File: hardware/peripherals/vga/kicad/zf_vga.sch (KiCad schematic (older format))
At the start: 34 parts, among them J1 Conn_02x04_Odd_Even, J2 Conn_02x13_Odd_Even, J3 DB15_Female, J4 DB9_Male, J5 DB9_Male, SW1 SW_DIP_x03, U1 4040, U10 74HC165, U11 AS6C6264, U12 74HC541, U13 74HC541, U14 74HC541, U2 4040, U3 GAL16V8, U4 GAL16V8, U5 74HC541, U6 74HC541, U7 74HC00, U8 74HC04, U9 74HC74, X1 CXO_DIP14

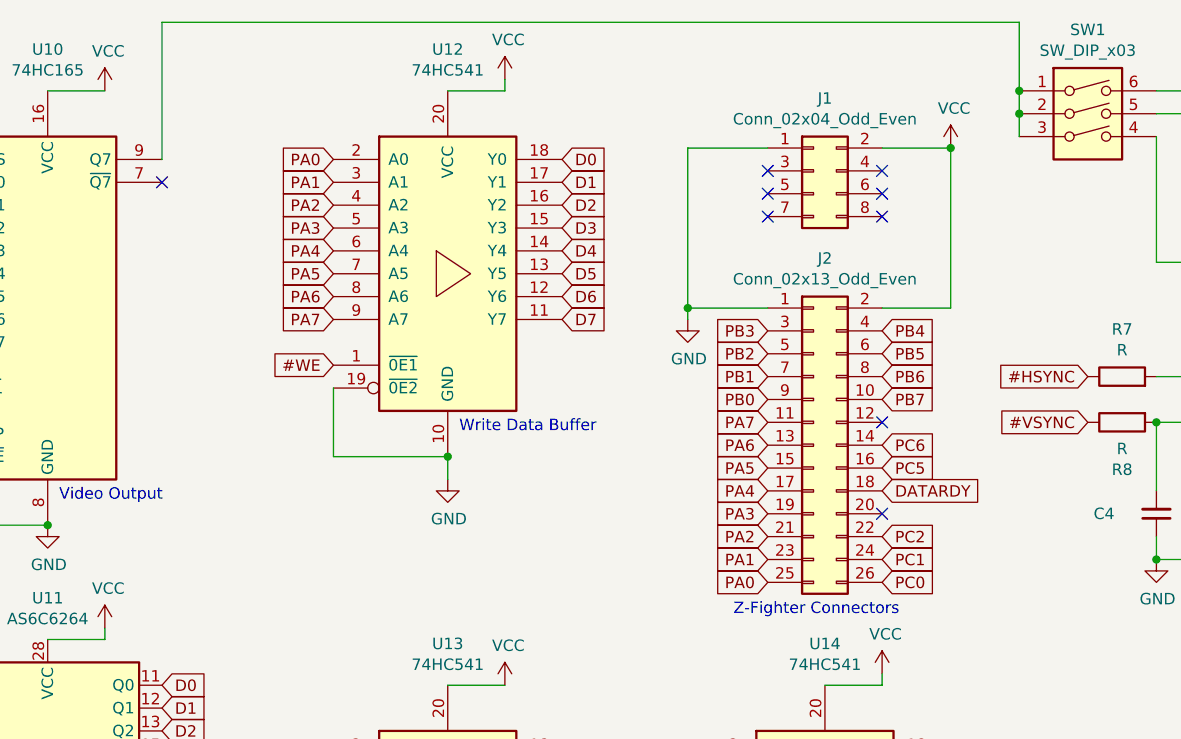
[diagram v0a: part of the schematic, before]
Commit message: Started PCB
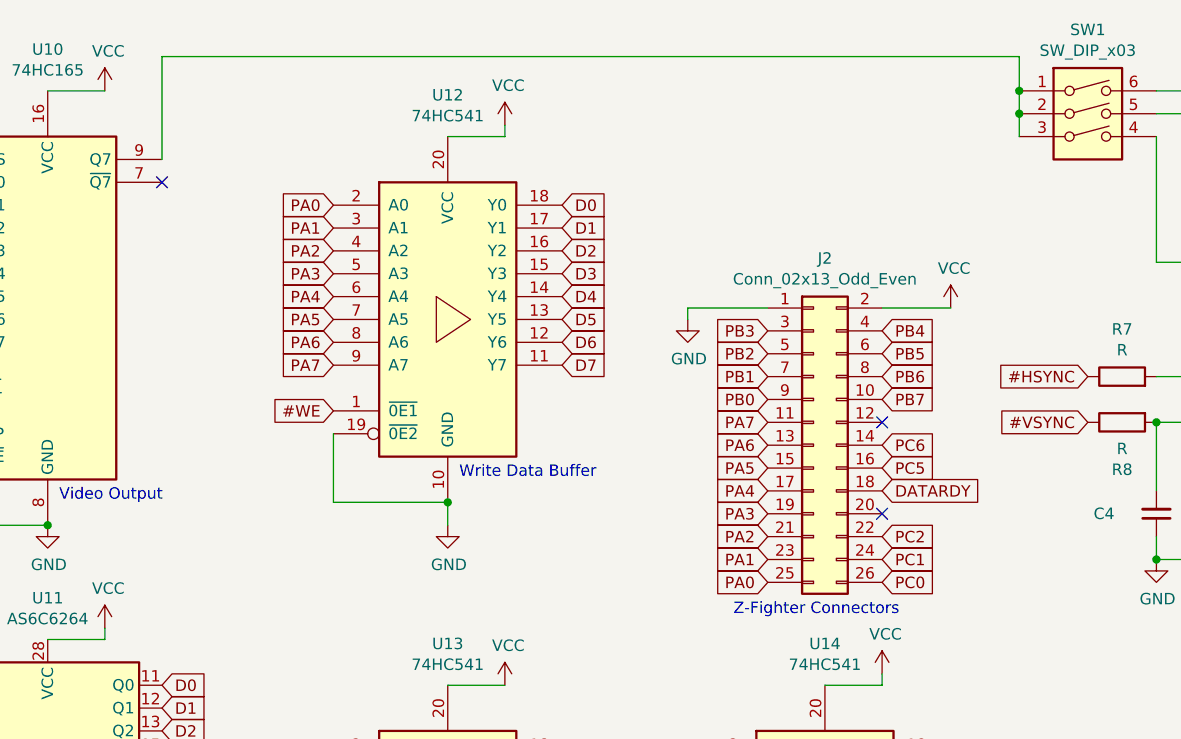
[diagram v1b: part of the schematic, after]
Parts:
- removed J1: Conn_02x04_Odd_Even, symbol Connector_Generic:Conn_02x04_Odd_Even
- C1, C2, C3, C4, C5: footprint (none) -> Capacitor_THT:C_Disc_D7.5mm_W2.5mm_P5.00mm
- J2: footprint (none) -> Connector_IDC:IDC-Header_2x13_P2.54mm_Vertical
- R1, R2, R3, R4, R5, R6, R7, R8: footprint (none) -> Resistor_THT:R_Axial_DIN0207_L6.3mm_D2.5mm_P7.62mm_Horizontal
- SW1: footprint (none) -> Button_Switch_THT:SW_DIP_SPSTx03_Slide_6.7x9.18mm_W7.62mm_P2.54mm_LowProfile
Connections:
- no-connect marks 35 -> 29
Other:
- moved on the sheet: U12

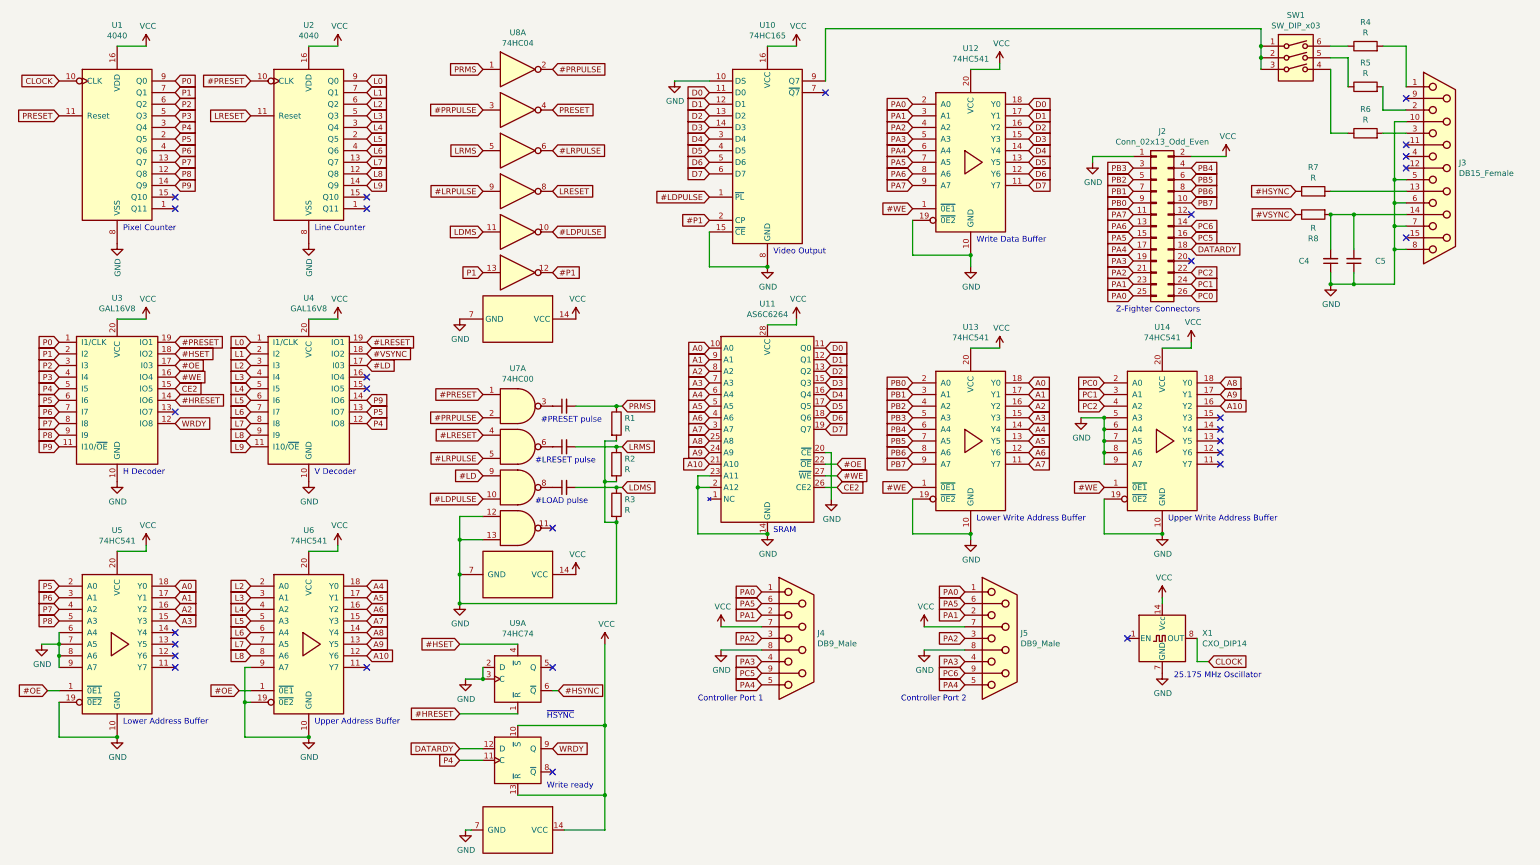
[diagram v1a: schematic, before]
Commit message: Bypass caps
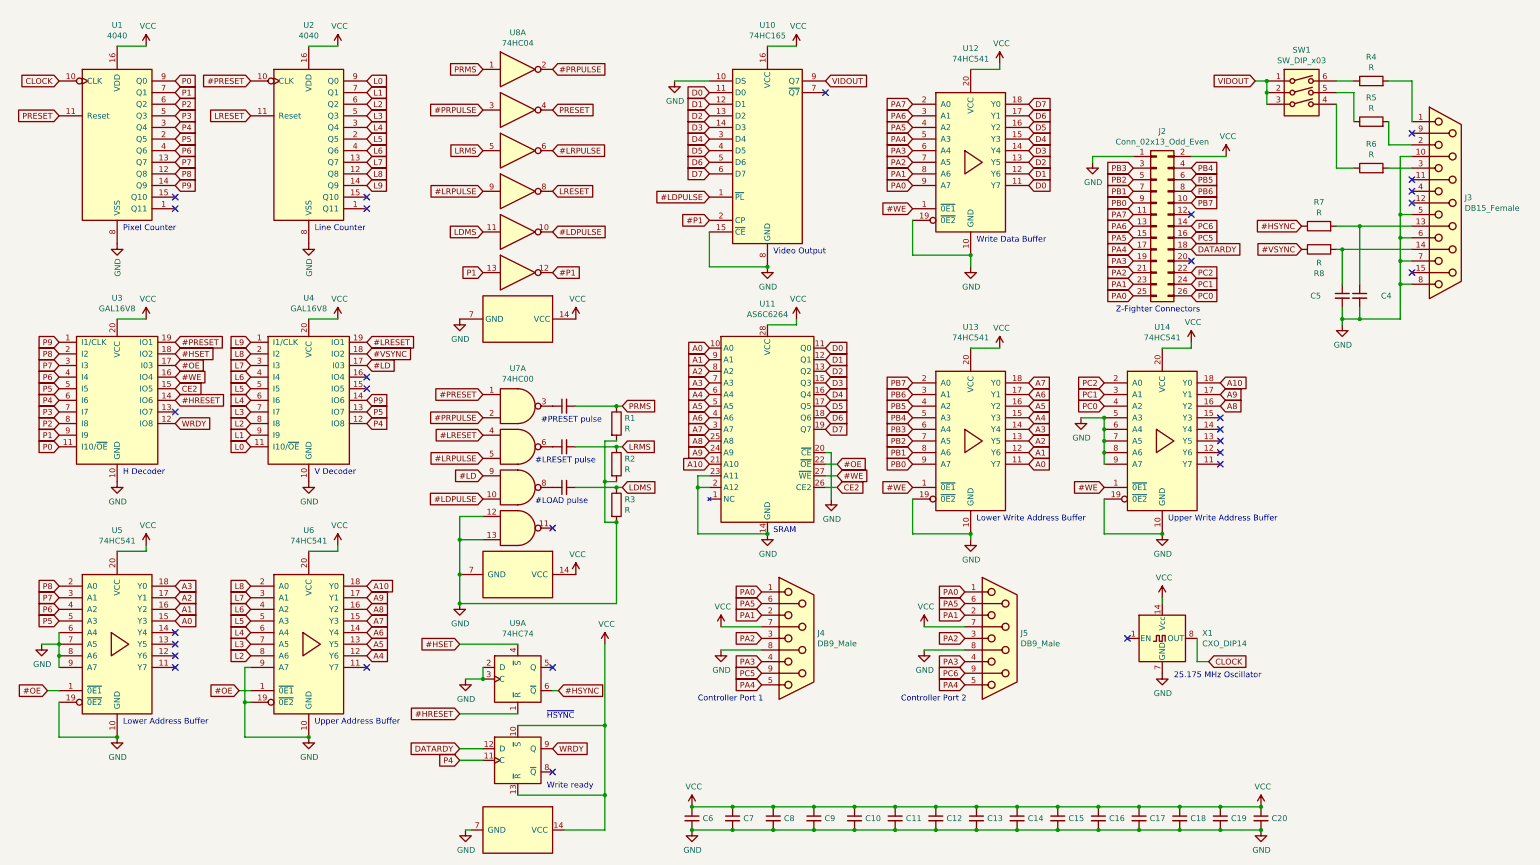
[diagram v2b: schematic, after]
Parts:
- added C10, C11, C12, C13, C14, C15, C16, C17, C18, C19, C20, C6, C7, C8, C9: 0.1uF, Capacitor_THT:C_Disc_D7.5mm_W2.5mm_P5.00mm, symbol Device:C_Small
- SW1: footprint Button_Switch_THT:SW_DIP_SPSTx03_Slide_6.7x9.18mm_W7.62mm_P2.54mm_LowProfile -> Package_DIP:DIP-6_W7.62mm_LongPads
- U1, U10, U2: footprint Package_DIP:DIP-16_W7.62mm -> Package_DIP:DIP-16_W7.62mm_LongPads
- U11: footprint Package_DIP:DIP-28_W15.24mm -> Package_DIP:DIP-28_W15.24mm_LongPads
- U12, U13, U14, U3, U4, U5, U6: footprint Package_DIP:DIP-20_W7.62mm -> Package_DIP:DIP-20_W7.62mm_LongPads
- X1: footprint Oscillator:Oscillator_DIP-14 -> Oscillator:Oscillator_DIP-14_LargePads
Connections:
- net A0: now also U13.11 (Y7), U5.15 (Y3); no longer U13.18 (Y0), U5.18 (Y0)
- net A1: now also U13.12 (Y6), U5.16 (Y2); no longer U13.17 (Y1), U5.17 (Y1)
- net A10: now also U14.18 (Y0), U6.18 (Y0); no longer U14.16 (Y2), U6.12 (Y6)
- net A2: now also U13.13 (Y5), U5.17 (Y1); no longer U13.16 (Y2), U5.16 (Y2)
- net A3: now also U13.14 (Y4), U5.18 (Y0); no longer U13.15 (Y3), U5.15 (Y3)
- net A4: now also U13.15 (Y3), U6.12 (Y6); no longer U13.14 (Y4), U6.18 (Y0)
- net A5: now also U13.16 (Y2), U6.13 (Y5); no longer U13.13 (Y5), U6.17 (Y1)
- net A6: now also U13.17 (Y1), U6.14 (Y4); no longer U13.12 (Y6), U6.16 (Y2)
- net A7: now also U13.18 (Y0); no longer U13.11 (Y7)
- net A8: now also U14.16 (Y2), U6.16 (Y2); no longer U14.18 (Y0), U6.14 (Y4)
- net A9: now also U6.17 (Y1); no longer U6.13 (Y5)
- net D0: now also U12.11 (Y7); no longer U12.18 (Y0)
- net D1: now also U12.12 (Y6); no longer U12.17 (Y1)
- net D2: now also U12.13 (Y5); no longer U12.16 (Y2)
- net D3: now also U12.14 (Y4); no longer U12.15 (Y3)
- net D4: now also U12.15 (Y3); no longer U12.14 (Y4)
- net D5: now also U12.16 (Y2); no longer U12.13 (Y5)
- net D6: now also U12.17 (Y1); no longer U12.12 (Y6)
- net D7: now also U12.18 (Y0); no longer U12.11 (Y7)
- net GND: now also C4.2, C5.2, C10.2, C11.2, C12.2, C13.2, C14.2, C15.2, C16.2, C17.2, C18.2, C19.2, C20.2, C6.2, C7.2, C8.2, C9.2; no longer C4.1, C5.1
- net L0: now also U4.11 (I10/~OE~); no longer U4.1 (I1/CLK)
- net L1: now also U4.9 (I9); no longer U4.2 (I2)
- net L2: now also U4.8 (I8), U6.8 (A6); no longer U4.3 (I3), U6.2 (A0)
- net L3: now also U4.7 (I7), U6.7 (A5); no longer U4.4 (I4), U6.3 (A1)
- net L4: now also U4.6 (I6), U6.6 (A4); no longer U4.5 (I5), U6.4 (A2)
- net L5: now also U4.5 (I5); no longer U4.6 (I6)
- net L6: now also U4.4 (I4), U6.4 (A2); no longer U4.7 (I7), U6.6 (A4)
- net L7: now also U4.3 (I3), U6.3 (A1); no longer U4.8 (I8), U6.7 (A5)
- net L8: now also U4.2 (I2), U6.2 (A0); no longer U4.9 (I9), U6.8 (A6)
- net L9: now also U4.1 (I1/CLK); no longer U4.11 (I10/~OE~)
- net P0: now also U3.11 (I10/~OE~); no longer U3.1 (I1/CLK)
- net P1: now also U3.9 (I9); no longer U3.2 (I2)
- net P2: now also U3.8 (I8); no longer U3.3 (I3)
- net P3: now also U3.7 (I7); no longer U3.4 (I4)
- net P4: now also U3.6 (I6); no longer U3.5 (I5)
- net P5: now also U3.5 (I5), U5.5 (A3); no longer U3.6 (I6), U5.2 (A0)
- net P6: now also U3.4 (I4), U5.4 (A2); no longer U3.7 (I7), U5.3 (A1)
- net P7: now also U3.3 (I3), U5.3 (A1); no longer U3.8 (I8), U5.4 (A2)
- net P8: now also U3.2 (I2), U5.2 (A0); no longer U3.9 (I9), U5.5 (A3)
- net P9: now also U3.1 (I1/CLK); no longer U3.11 (I10/~OE~)
- net PA0: now also U12.9 (A7); no longer U12.2 (A0)
- net PA1: now also U12.8 (A6); no longer U12.3 (A1)
- net PA2: now also U12.7 (A5); no longer U12.4 (A2)
- net PA3: now also U12.6 (A4); no longer U12.5 (A3)
- net PA4: now also U12.5 (A3); no longer U12.6 (A4)
- net PA5: now also U12.4 (A2); no longer U12.7 (A5)
- net PA6: now also U12.3 (A1); no longer U12.8 (A6)
- net PA7: now also U12.2 (A0); no longer U12.9 (A7)
- net PB0: now also U13.9 (A7); no longer U13.2 (A0)
- net PB1: now also U13.8 (A6); no longer U13.3 (A1)
- net PB2: now also U13.7 (A5); no longer U13.4 (A2)
- net PB3: now also U13.6 (A4); no longer U13.5 (A3)
- net PB4: now also U13.5 (A3); no longer U13.6 (A4)
- net PB5: now also U13.4 (A2); no longer U13.7 (A5)
- net PB6: now also U13.3 (A1); no longer U13.8 (A6)
- net PB7: now also U13.2 (A0); no longer U13.9 (A7)
- net PC0: now also U14.4 (A2); no longer U14.2 (A0)
- net PC2: now also U14.2 (A0); no longer U14.4 (A2)
- net VCC: now also C10.1, C11.1, C12.1, C13.1, C14.1, C15.1, C16.1, C17.1, C18.1, C19.1, C20.1, C6.1, C7.1, C8.1, C9.1
- net VIDOUT: now reaches SW1.1, SW1.2, SW1.3, U10.9 (Q7)
- net at J3.13 (P13), R7.2: now also C4.1
- net at J3.14 (P14), R8.2: now also C5.1; no longer C4.2, C5.2
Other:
- moved on the sheet: C4, C5, J3, R4, R5, R6, R7, R8, SW1
